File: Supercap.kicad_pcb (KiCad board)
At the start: 4 copper layers, 151.8 x 70 mm, 69 parts, among them IC1 NCP5109ADR2G, IC2 NCP5109ADR2G, J1 XT30, J2 XT30, J2-J1 Conn_01x10, J3 Conn_01x01, J3-J1 Conn_01x10, J4 Conn_01x01, P7803B-1000R1 P7803B-1000, P7812B-1000R1 490-P7812B-1000, U1 TLV2372, U2 TLV2372, U4 ACS71240KEXBLT-010B3, U6 LP-MSPM0G3507

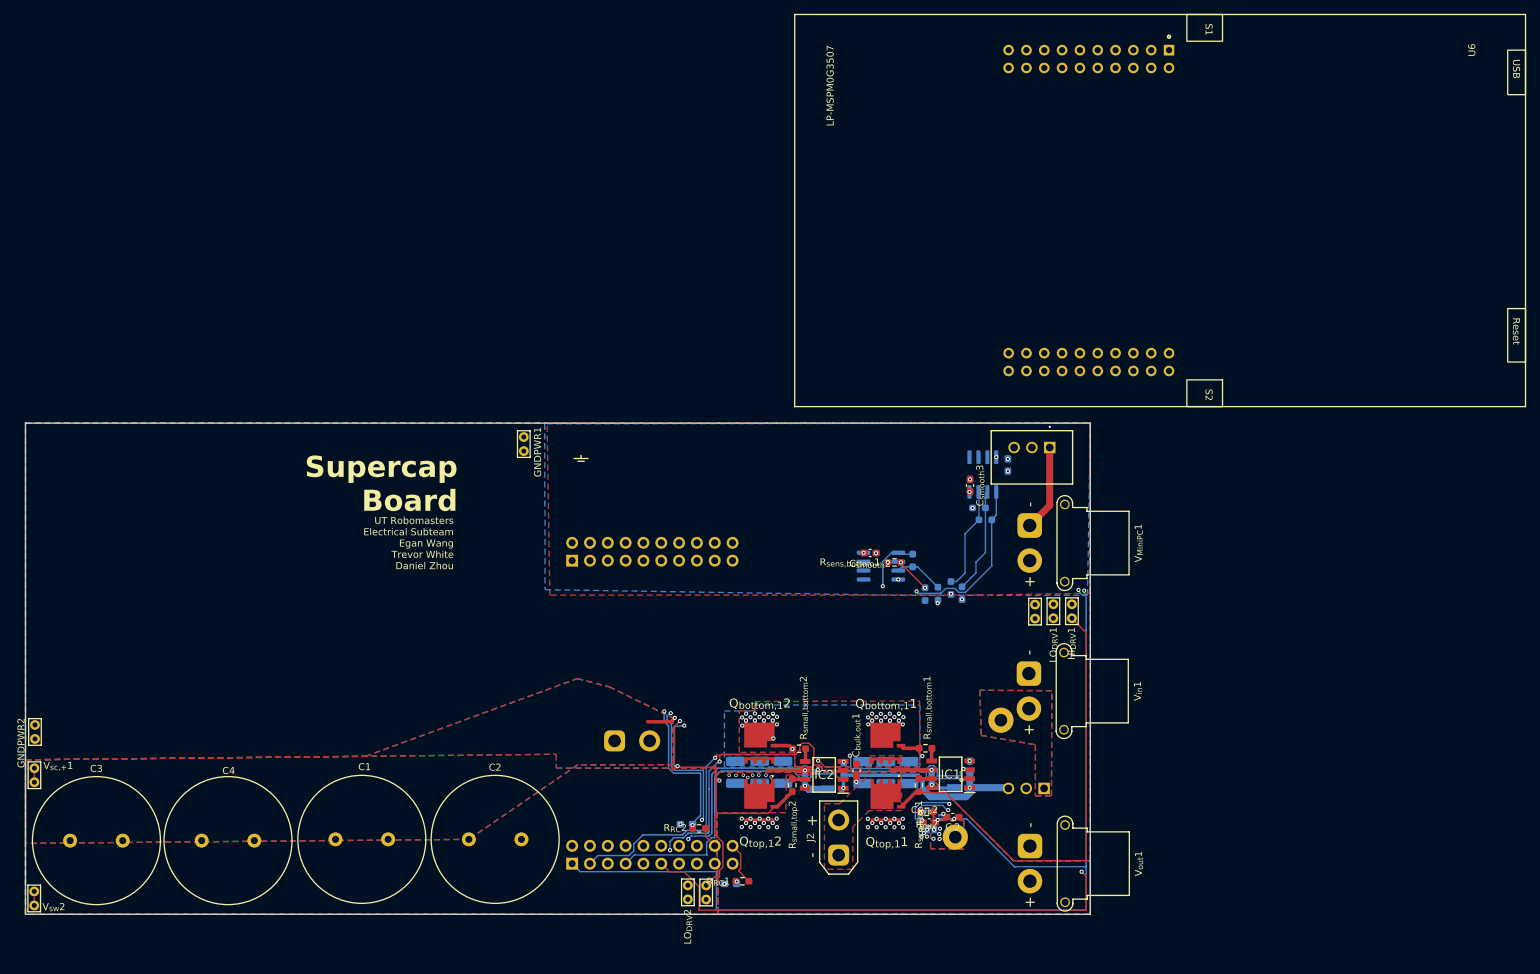
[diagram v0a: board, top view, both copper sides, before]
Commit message: starting on V3 :) yipee. finished pours and stuff
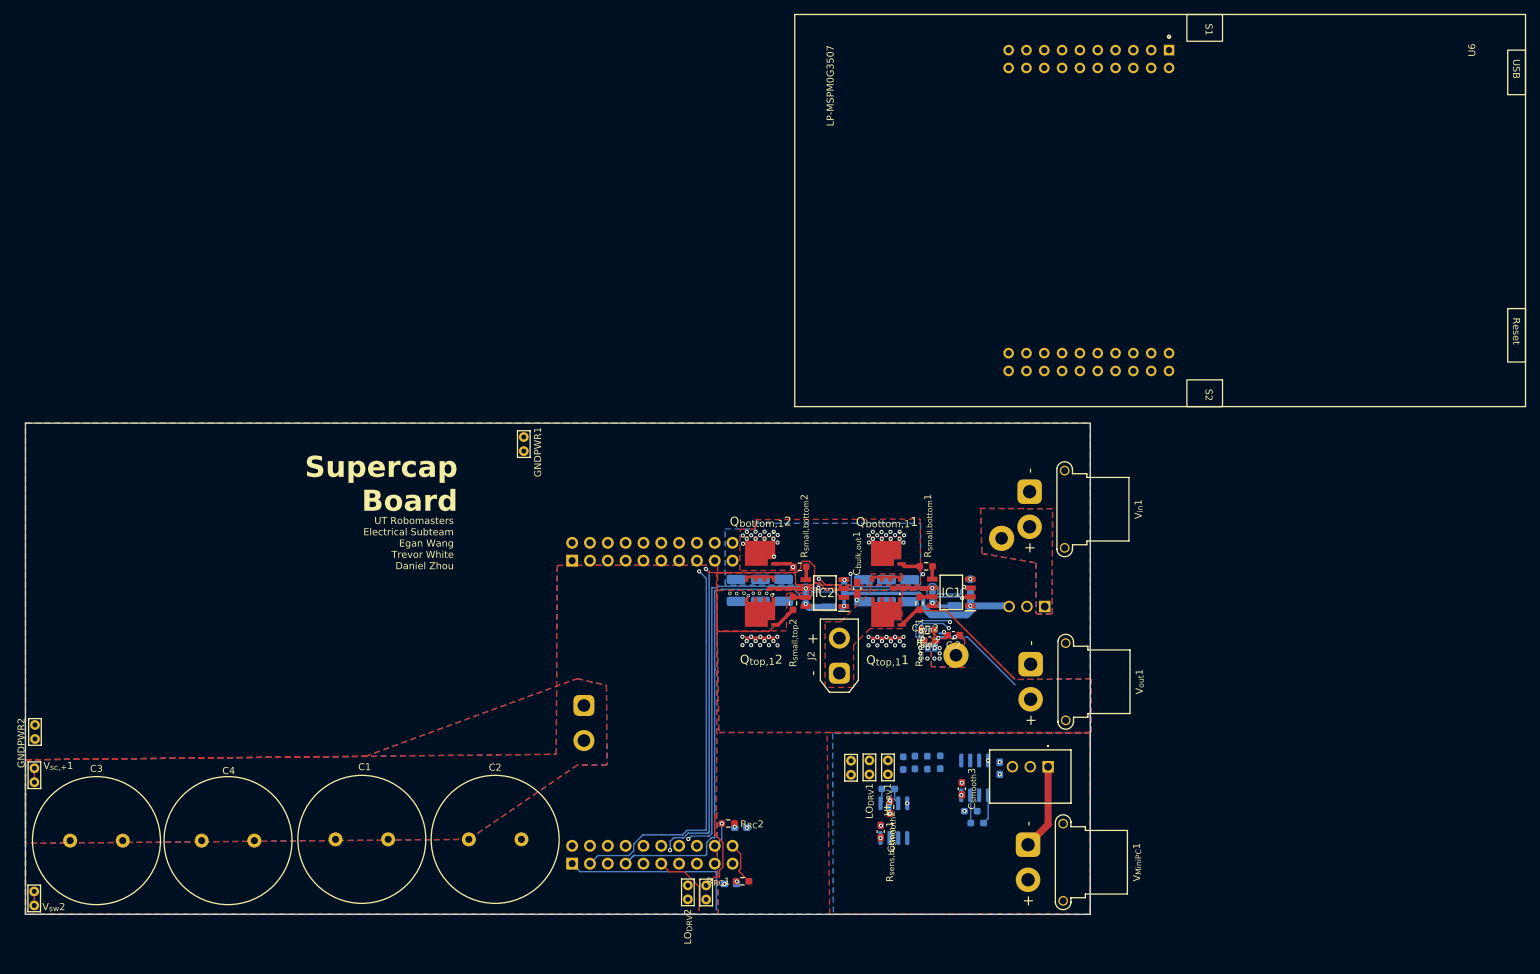
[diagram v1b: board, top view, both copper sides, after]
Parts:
- moved P7803B-1000R1 45.5 mm to (183.3, 120.2)
- moved V_{MiniPC}1 45.5 mm to (180.4, 131.3)
- moved C_{smooth}3 43.2 mm to (171.0, 123.4)
- moved R4 43.2 mm to (173.2, 128.3)
- moved U1 43.2 mm to (172.8, 121.8)
- moved C_{smooth}1 43.2 mm to (176.4, 120.5)
- moved R3 43.2 mm to (172.3, 126.6)
- moved C_{smooth}2 39.7 mm to (159.4, 129.5), turned to 90 degrees
- moved U2 36.3 mm to (161.3, 127.9), turned to -90 degrees
- moved R_{sens,bottom}1 34.9 mm to (160.8, 126.0), turned to 90 degrees
- moved LO_{DRV}1 34.4 mm to (157.8, 121.3)
- moved V_{sw}1 34.4 mm to (155.2, 121.4)
- moved HI_{DRV}1 34.4 mm to (160.5, 121.3)
- moved R_{sens,bottom}2 32.7 mm to (160.5, 123.4), turned to 180 degrees
- moved J2 25.9 mm to (153.5, 106.9)
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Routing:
- net /Control/+3V3: track 152.2 -> 42.9 mm, vias 7 -> 6
- net GND: track 160.1 -> 66.4 mm, vias 11 -> 10
- net /Control/V_{sc,sens}: track 96.8 -> 4.24 mm, vias 4 -> 1
- net /Control/F_bat: track 96.2 -> 25.3 mm
- net /Control/I_bat: track 95.0 -> 28.0 mm, vias 2 -> 1
- net /Control/V_{bat,sens}: track 67.8 -> 2.09 mm, vias 3 -> 1
- net /Control/I_{bat,out+}: track 59.6 -> 0.00 mm, vias 38 -> 34
- net /Voltage Converter/V_{sw,2}: track 63.5 -> 7.37 mm, vias 11 -> 9
- net /Control/V_{sc,+}: track 53.1 -> 2.00 mm, vias 2 -> 0
- net /Voltage Converter/V_{sw,1}: track 76.3 -> 25.7 mm
- net /Voltage Converter/HI_DRV_{1}: track 68.8 -> 23.1 mm
- net /Voltage Converter/LO_DRV_{1}: track 74.1 -> 36.0 mm
- net /Control/PA25: track 51.6 -> 80.3 mm
- net /Control/PB9: track 44.3 -> 72.6 mm
- net /Control/PA8: track 64.0 -> 92.1 mm
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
